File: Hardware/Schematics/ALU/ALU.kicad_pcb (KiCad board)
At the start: 4 copper layers, 188.4 x 135.2 mm, 54 parts, among them J1 Conn_01x10, J2 Conn_01x10, J3 Conn_02x05_Counter_Clockwise, J4 Conn_01x10, J5 Conn_02x05_Counter_Clockwise, U1 74LS113, U10 74LS83, U11 74LS83, U12 74LS245, U13 74LS00, U14 74LS00, U15 74LS245, U16 74LS245, U17 74LS245, U18 74LS245, U19 74LS86, U2 74LS32, U20 74LS86, U21 74LS32, U22 74LS08, U3 74LS113, U4 74LS86, U5 74LS04, U6 74LS86, U7 74LS32, U8 74LS245, U9 74LS245

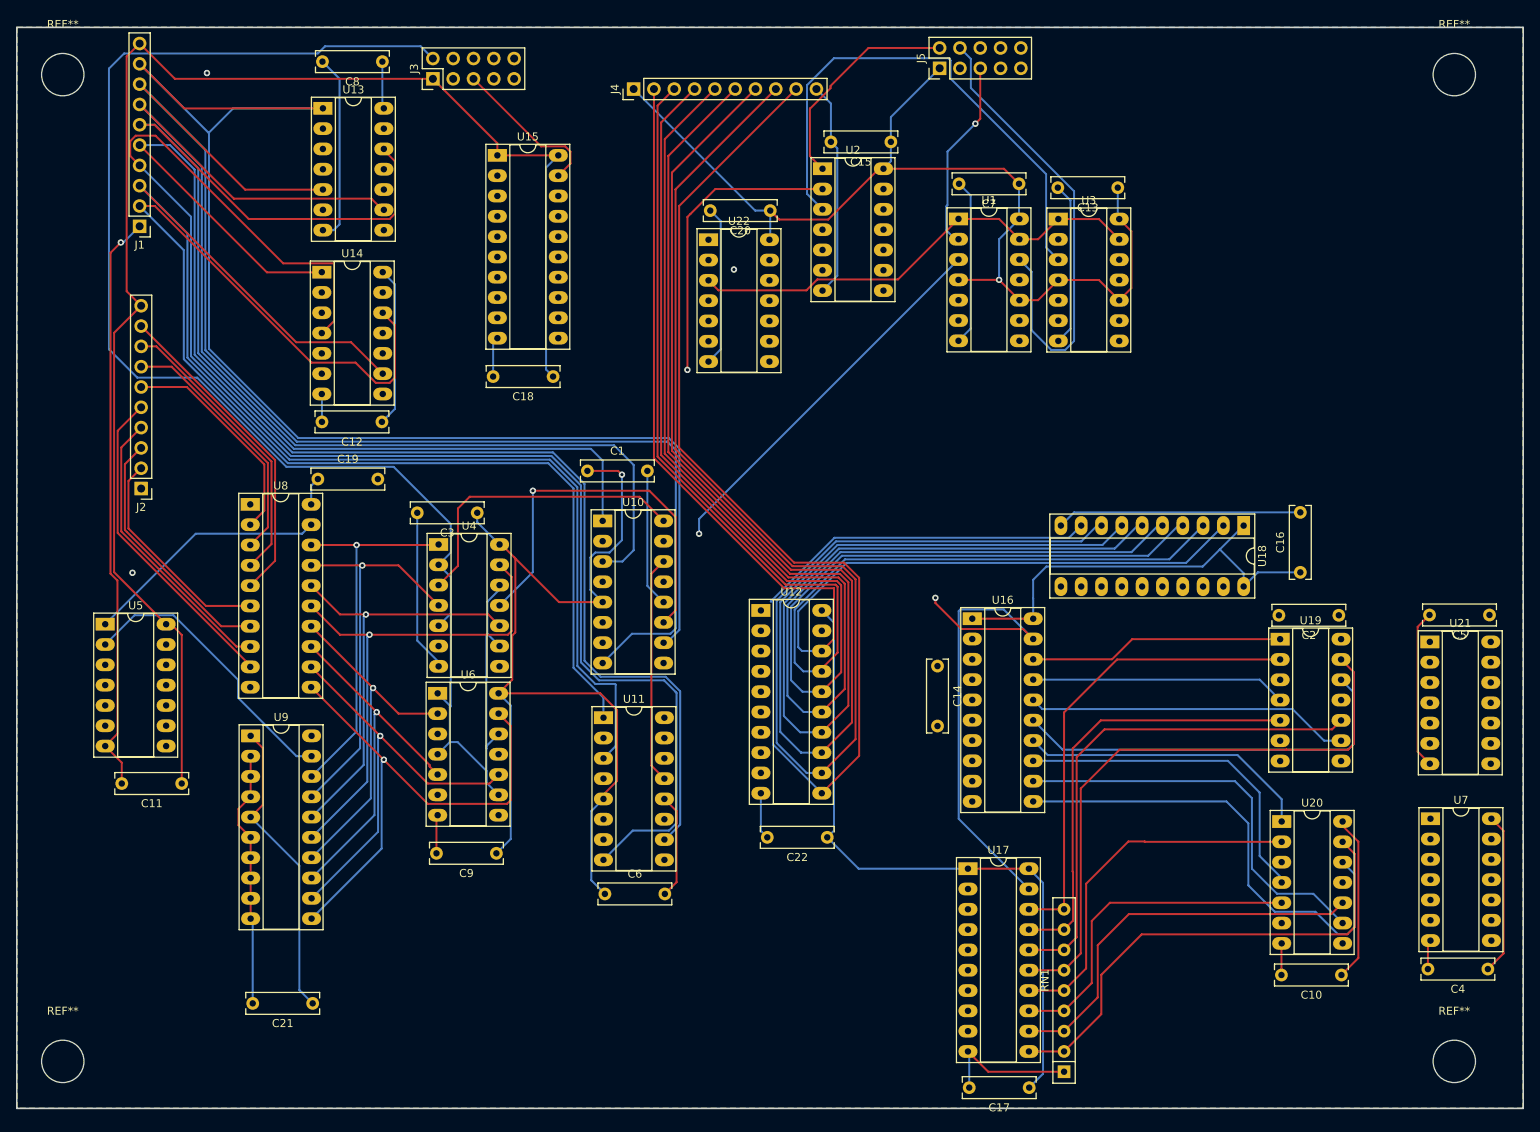
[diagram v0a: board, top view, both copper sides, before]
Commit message: Updated Schematics
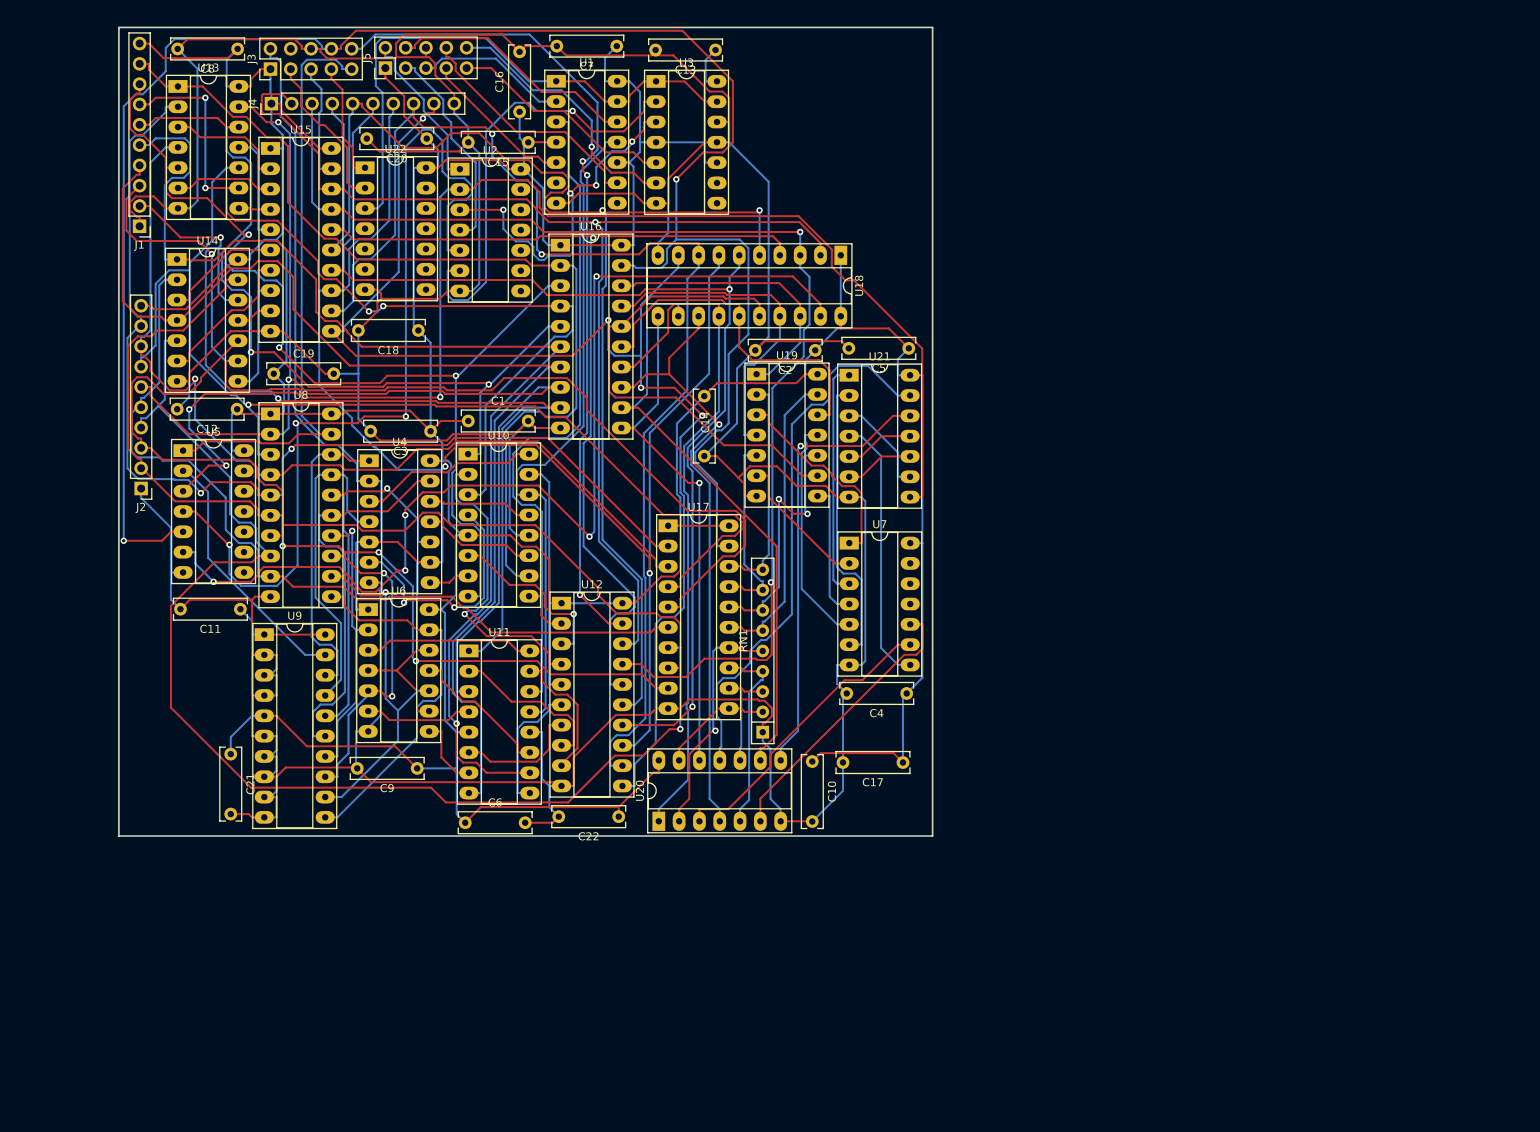
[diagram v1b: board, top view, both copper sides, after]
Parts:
- removed REF** (x4): MountingHole_5.3mm_M5, MountingHole:MountingHole_5.3mm_M5
- moved C16 113.4 mm to (89.0, 30.5)
- moved C4 80.5 mm to (137.4, 103.2)
- moved U7 80.5 mm to (130.2, 84.4)
- moved U21 79.9 mm to (130.2, 63.4)
- moved C5 79.9 mm to (137.7, 60.0)
- moved U20 77.9 mm to (106.4, 119.2), turned to 90 degrees
- moved C2 73.4 mm to (126.0, 60.3)
- moved U19 73.4 mm to (118.7, 63.3)
- moved C10 71.4 mm to (125.6, 111.7), turned to -90 degrees
- moved U16 69.5 mm to (94.1, 47.1)
- moved J5 69.3 mm to (72.2, 25.0)
- moved U18 60.7 mm to (129.2, 48.4)
- moved U17 57.0 mm to (107.6, 82.2)
- moved RN1 56.8 mm to (119.4, 108.1)
- moved C13 53.2 mm to (113.5, 22.7)
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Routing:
- net VCC: track 992.1 -> 627.8 mm, vias 2 -> 0
- net /Compare/RD != RS: track 498.7 -> 165.7 mm, vias 2 -> 3
- net /Adder/RD_{0}: track 421.9 -> 118.0 mm
- net /Adder/RD_{1}: track 408.0 -> 125.4 mm, vias 0 -> 3
- net /Adder/RD_{2}: track 383.9 -> 107.3 mm, vias 0 -> 4
- net GND: track 393.6 -> 666.3 mm, vias 1 -> 0
- net /Adder/RD_{3}: track 374.0 -> 103.4 mm, vias 0 -> 2
- net /Adder/RD_{5}: track 408.2 -> 148.7 mm
- net /Adder/RD_{4}: track 396.1 -> 149.7 mm, vias 0 -> 1
- net /Adder/RD_{6}: track 368.6 -> 128.2 mm, vias 0 -> 1
- net /Adder/RD_{7}: track 358.1 -> 122.9 mm, vias 0 -> 2
- net /Compare/RD == RS: track 269.6 -> 113.2 mm, vias 0 -> 3
- net /Adder/RS_{4}: track 253.7 -> 106.8 mm
- net /Adder/RS_{7}: track 255.5 -> 119.3 mm, vias 0 -> 3
- net /Adder/RS_{1}: track 251.5 -> 115.7 mm, vias 0 -> 1
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- removed copper zone on B.Cu, net GND
- removed copper zone on F.Cu, net GND
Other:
- board size 188.4 x 135.2 mm -> 101.8 x 101.1 mm
- copper layers 4 -> 2
